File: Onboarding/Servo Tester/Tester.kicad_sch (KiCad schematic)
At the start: 6 parts, among them SW1 RotaryEncoder_Switch, U1 PCF8551ATT_AJ, U3 ATTINY204-SSNR, U4 AP2205-33Y-13, U5 VIM-878-DP-FC-S-LV

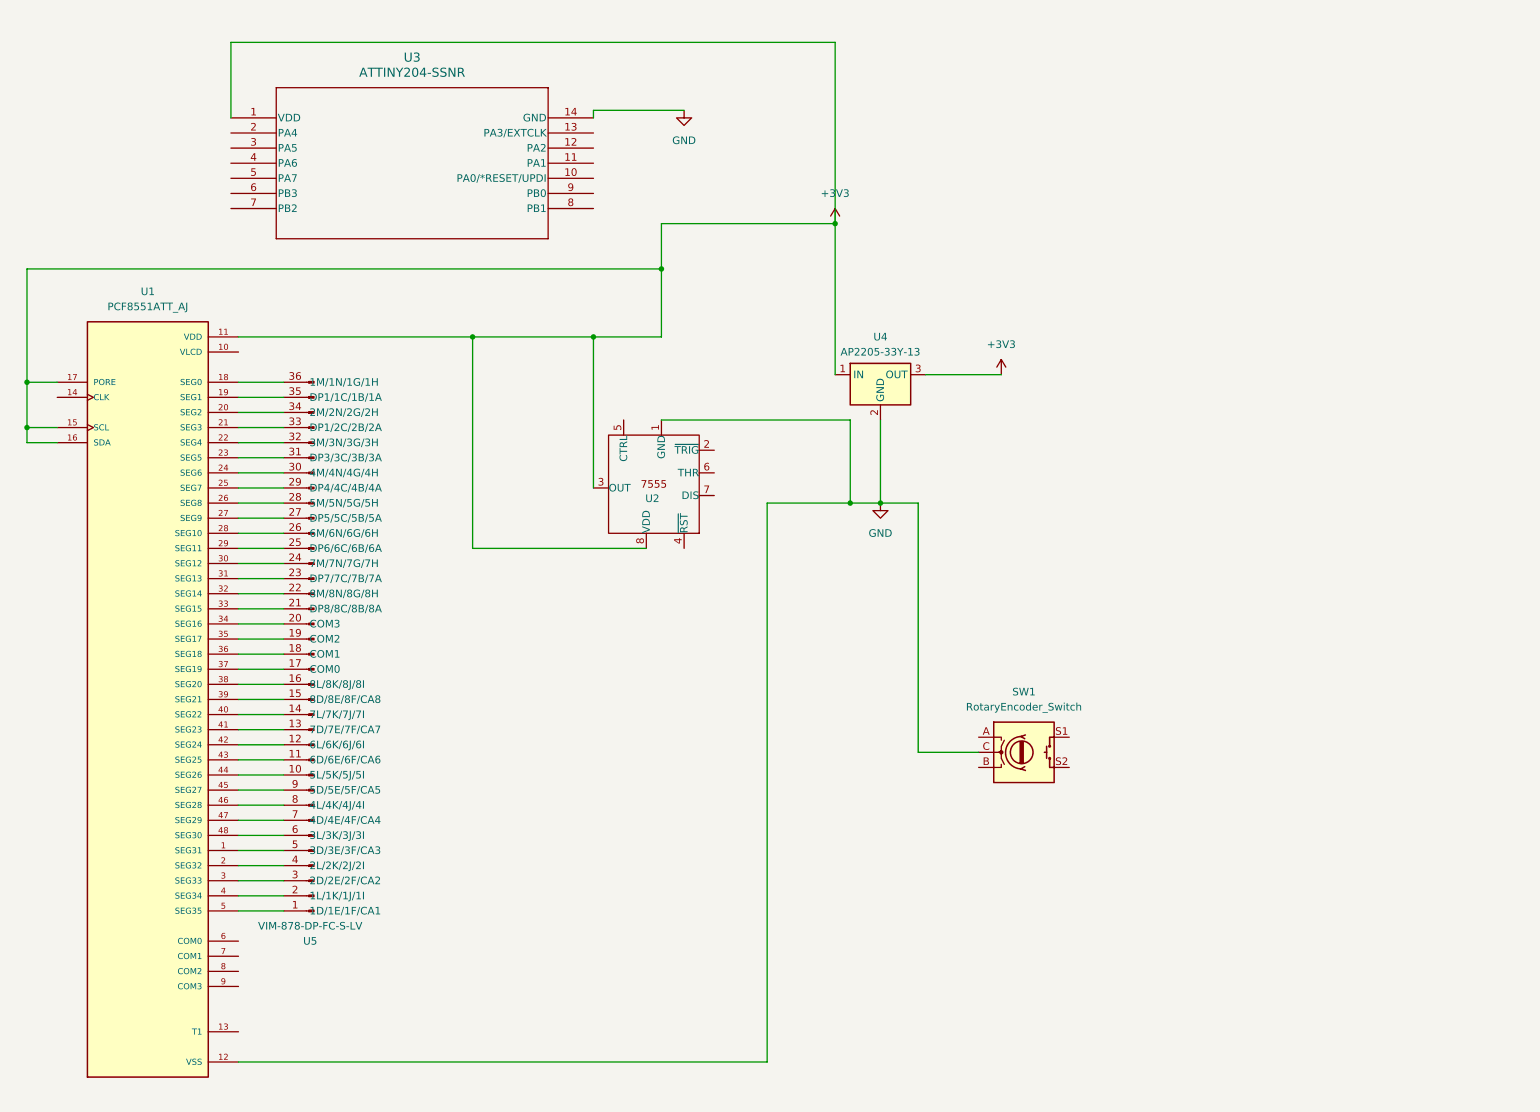
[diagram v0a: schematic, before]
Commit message: Update Tester.kicad_sch
Progress has been made.
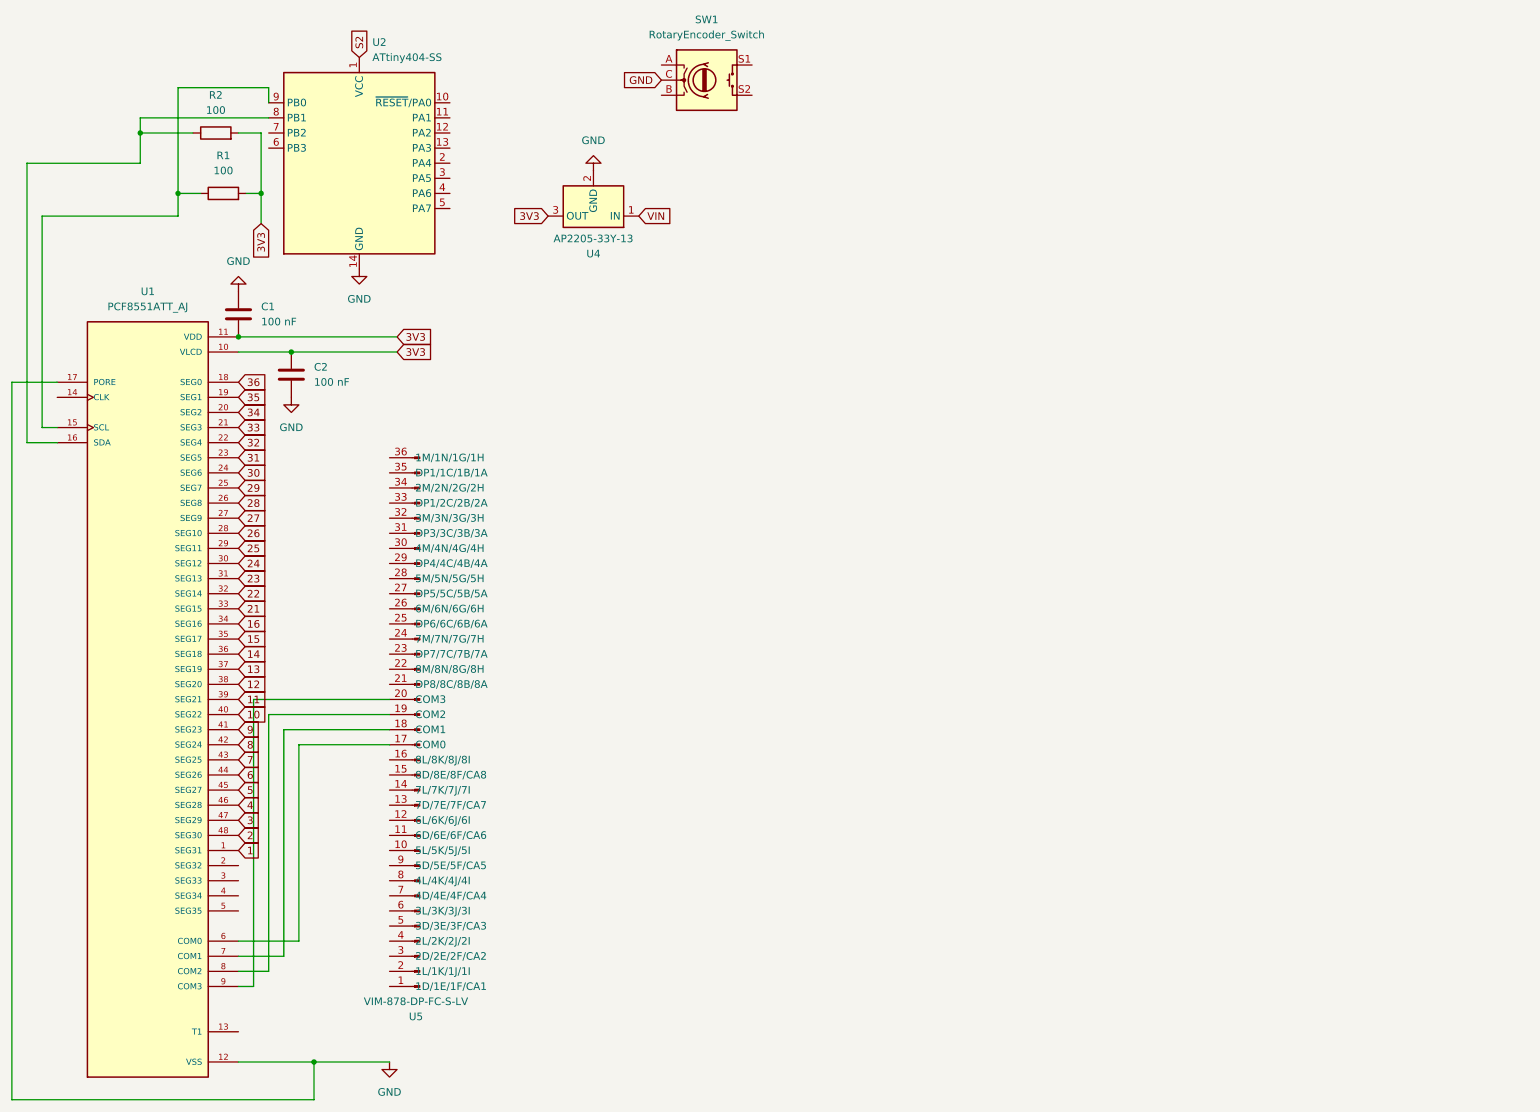
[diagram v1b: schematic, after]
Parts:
- removed U2: ~, symbol NewSymbolLibrary:7555
- removed U3: ATTINY204-SSNR, SOIC14_SL_MCH, symbol ServoTester:ATTINY204-SSNR
- added C1, C2: 100 nF, symbol Device:C
- added R1, R2: 100, symbol Device:R
- added U2: ATtiny404-SS, Package_SO:SOIC-14_3.9x8.7mm_P1.27mm, symbol servo_tester_onboarding:ATtiny404-SS
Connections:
- net GND: now also U1.17 (PORE), C1.1, C2.2, U2.14 (GND)
- net at U5.5 (3D/3E/3F/CA3): no longer U1.1 (SEG31)
- net 3V3: now reaches U1.10 (VLCD)
- net 3V3: now also U1.11 (VDD), U4.3 (OUT), C1.2, C2.1, R1.2, R2.2
- net at U5.36 (1M/1N/1G/1H): no longer U1.18 (SEG0)
- net at U5.35 (DP1/1C/1B/1A): no longer U1.19 (SEG1)
- net at U1.2 (SEG32): no longer U5.4 (2L/2K/2J/2I)
- net at U5.34 (2M/2N/2G/2H): no longer U1.20 (SEG2)
- net at U5.33 (DP1/2C/2B/2A): no longer U1.21 (SEG3)
- net at U5.32 (3M/3N/3G/3H): no longer U1.22 (SEG4)
- net at U5.31 (DP3/3C/3B/3A): no longer U1.23 (SEG5)
- net at U5.30 (4M/4N/4G/4H): no longer U1.24 (SEG6)
- net at U5.29 (DP4/4C/4B/4A): no longer U1.25 (SEG7)
- net at U5.28 (5M/5N/5G/5H): no longer U1.26 (SEG8)
- net at U5.27 (DP5/5C/5B/5A): no longer U1.27 (SEG9)
- net at U5.26 (6M/6N/6G/6H): no longer U1.28 (SEG10)
- net at U5.25 (DP6/6C/6B/6A): no longer U1.29 (SEG11)
- net at U1.3 (SEG33): no longer U5.3 (2D/2E/2F/CA2)
- net at U5.24 (7M/7N/7G/7H): no longer U1.30 (SEG12)
- net at U5.23 (DP7/7C/7B/7A): no longer U1.31 (SEG13)
- net at U5.22 (8M/8N/8G/8H): no longer U1.32 (SEG14)
- net at U5.21 (DP8/8C/8B/8A): no longer U1.33 (SEG15)
- net at U5.20 (COM3): now also U1.9 (COM3); no longer U1.34 (SEG16)
- net at U5.19 (COM2): now also U1.8 (COM2); no longer U1.35 (SEG17)
- net at U5.18 (COM1): now also U1.7 (COM1); no longer U1.36 (SEG18)
- net at U5.17 (COM0): now also U1.6 (COM0); no longer U1.37 (SEG19)
- net at U5.16 (8L/8K/8J/8I): no longer U1.38 (SEG20)
- net at U5.15 (8D/8E/8F/CA8): no longer U1.39 (SEG21)
- net at U1.4 (SEG34): no longer U5.2 (1L/1K/1J/1I)
- net at U5.14 (7L/7K/7J/7I): no longer U1.40 (SEG22)
- net at U5.13 (7D/7E/7F/CA7): no longer U1.41 (SEG23)
- net at U5.12 (6L/6K/6J/6I): no longer U1.42 (SEG24)
- net at U5.11 (6D/6E/6F/CA6): no longer U1.43 (SEG25)
- net at U5.10 (5L/5K/5J/5I): no longer U1.44 (SEG26)
- net at U5.9 (5D/5E/5F/CA5): no longer U1.45 (SEG27)
- net at U5.8 (4L/4K/4J/4I): no longer U1.46 (SEG28)
- net at U5.7 (4D/4E/4F/CA4): no longer U1.47 (SEG29)
- net at U5.6 (3L/3K/3J/3I): no longer U1.48 (SEG30)
- net at U1.5 (SEG35): no longer U5.1 (1D/1E/1F/CA1)
- removed net +3V3: U1.11 (VDD), U1.15 (SCL), U1.16 (SDA), U1.17 (PORE), U4.1 (IN), U4.3 (OUT)
- new net: R2.1, U1.16 (SDA), U2.8 (PB1)
- new net: R1.1, U1.15 (SCL), U2.9 (PB0)
- new net 1: U1.1 (SEG31)
- new net 10: U1.40 (SEG22)
- new net 11: U1.39 (SEG21)
- new net 12: U1.38 (SEG20)
- new net 13: U1.37 (SEG19)
- new net 14: U1.36 (SEG18)
- new net 15: U1.35 (SEG17)
- new net 16: U1.34 (SEG16)
- new net 2: U1.48 (SEG30)
- new net 21: U1.33 (SEG15)
- new net 22: U1.32 (SEG14)
- new net 23: U1.31 (SEG13)
- new net 24: U1.30 (SEG12)
- new net 25: U1.29 (SEG11)
- new net 26: U1.28 (SEG10)
- new net 27: U1.27 (SEG9)
- new net 28: U1.26 (SEG8)
- new net 29: U1.25 (SEG7)
- new net 3: U1.47 (SEG29)
- new net 30: U1.24 (SEG6)
- new net 31: U1.23 (SEG5)
- new net 32: U1.22 (SEG4)
- new net 33: U1.21 (SEG3)
- new net 34: U1.20 (SEG2)
- new net 35: U1.19 (SEG1)
- new net 36: U1.18 (SEG0)
- new net 4: U1.46 (SEG28)
- new net 5: U1.45 (SEG27)
- new net 6: U1.44 (SEG26)
- new net 7: U1.43 (SEG25)
- new net 8: U1.42 (SEG24)
- new net 9: U1.41 (SEG23)
- new net S2: U2.1 (VCC)
- new net VIN: U4.1 (IN)
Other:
- moved on the sheet: SW1, U4, U5

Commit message: Test_bat
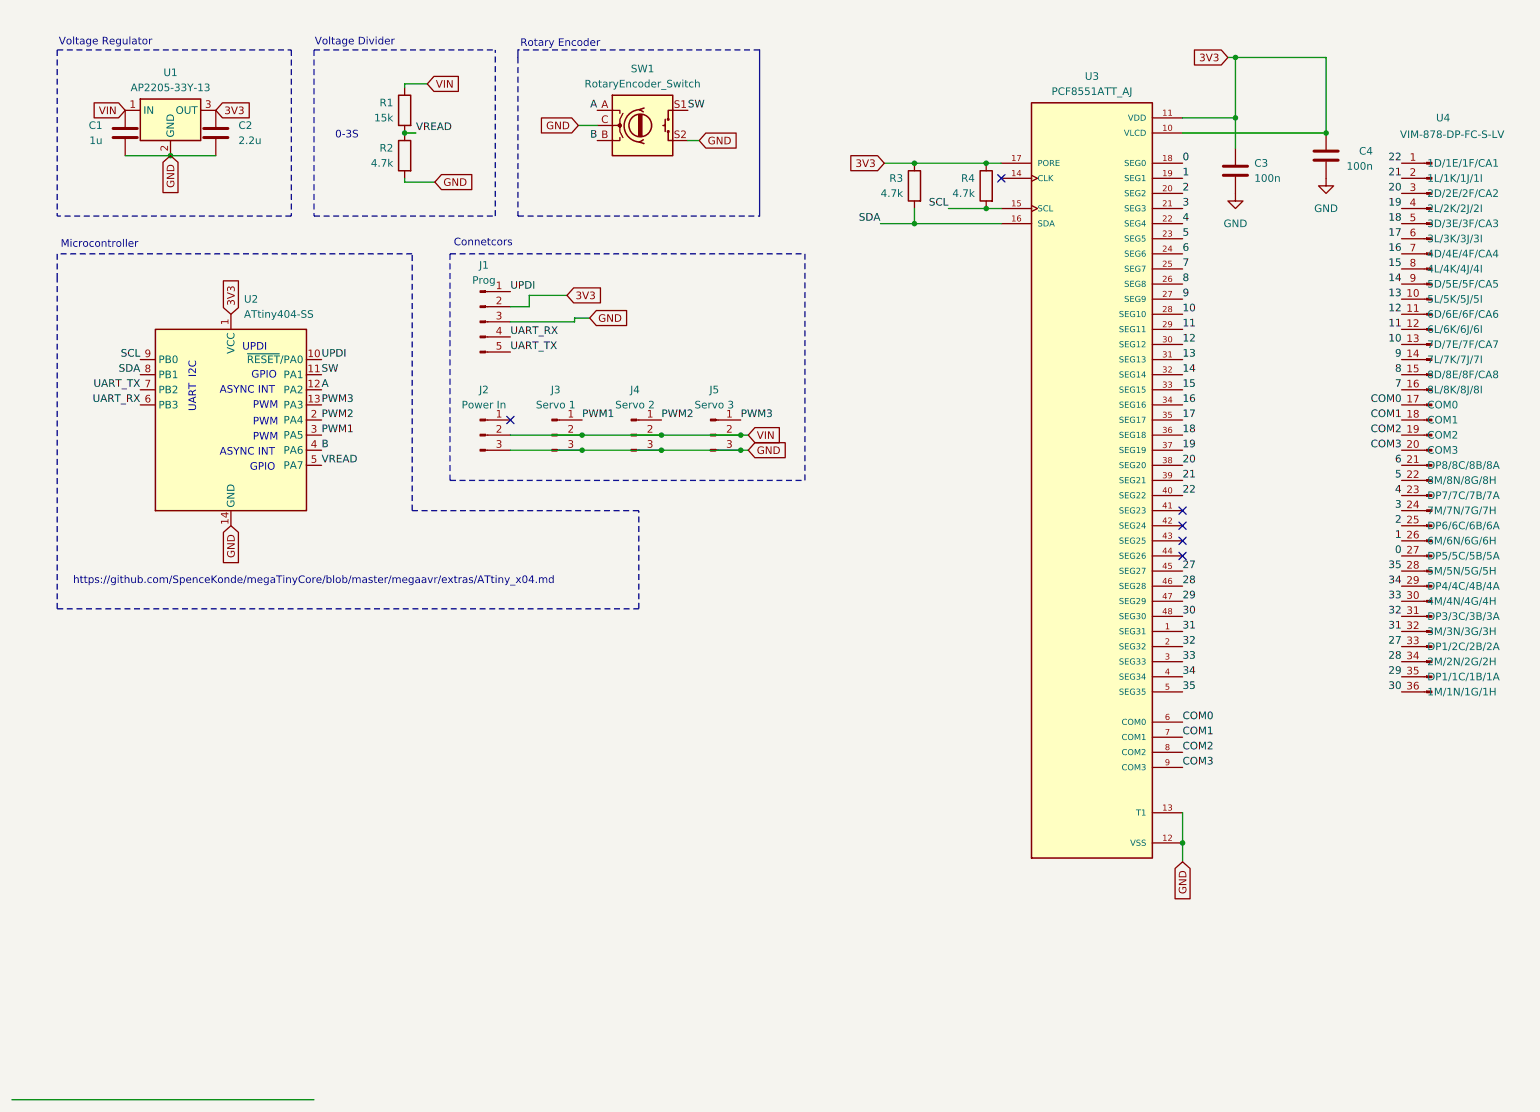
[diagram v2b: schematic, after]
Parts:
- removed SW1: RotaryEncoder_Switch, Rotary_Encoder:RotaryEncoder_Bourns_Vertical_PEC12R-3xxxF-Sxxxx, symbol servo_tester_onboarding:RotaryEncoder_Switch
- removed U1: PCF8551ATT_AJ, servo_tester:SOP50P810X120-48N, symbol servo_tester_onboarding:PCF8551ATT_AJ
- removed U2: ATtiny404-SS, Package_SO:SOIC-14_3.9x8.7mm_P1.27mm, symbol servo_tester_onboarding:ATtiny404-SS
- removed U4: AP2205-33Y-13, Package_TO_SOT_SMD:SOT-89-3_Handsoldering, symbol servo_tester_onboarding:AP2205-33Y-13
- removed U5: VIM-878-DP-FC-S-LV, symbol servo_tester_onboarding:VIM-878-DP
- added C3, C4: 100n, Capacitor_SMD:C_0603_1608Metric_Pad1.08x0.95mm_HandSolder, symbol Device:C
- added J1: Prog, Connector_PinSocket_2.54mm:PinSocket_1x05_P2.54mm_Vertical, symbol Connector:Conn_01x05_Pin
- added J2: Power In, Connector_PinSocket_2.54mm:PinSocket_1x03_P2.54mm_Vertical, symbol Connector:Conn_01x03_Pin
- added J3: Servo 1, Connector_PinSocket_2.54mm:PinSocket_1x03_P2.54mm_Vertical, symbol Connector:Conn_01x03_Pin
- added J4: Servo 2, Connector_PinSocket_2.54mm:PinSocket_1x03_P2.54mm_Vertical, symbol Connector:Conn_01x03_Pin
- added J5: Servo 3, Connector_PinSocket_2.54mm:PinSocket_1x03_P2.54mm_Vertical, symbol Connector:Conn_01x03_Pin
- added R3, R4: 4.7k, Resistor_SMD:R_0603_1608Metric_Pad0.98x0.95mm_HandSolder, symbol Device:R
- added SW1: RotaryEncoder_Switch, Rotary_Encoder:RotaryEncoder_Bourns_Vertical_PEC12R-3x17F-Sxxxx, symbol Device:RotaryEncoder_Switch
- added U1: AP2205-33Y-13, Package_TO_SOT_SMD:SOT-89-3_Handsoldering, symbol servo_tester:AP2205-33Y-13
- added U2: ATtiny404-SS, Package_SO:SOIC-14_3.9x8.7mm_P1.27mm, symbol MCU_Microchip_ATtiny:ATtiny404-SS
- added U3: PCF8551ATT_AJ, servo_tester:SOP50P810X120-48N, symbol servo_tester:PCF8551ATT_AJ
- added U4: VIM-878-DP-FC-S-LV, servo_tester:VIM-878-DP, symbol servo_tester:VIM-878-DP
- C1: value 100 nF -> 1u; footprint (none) -> Capacitor_SMD:C_0603_1608Metric_Pad1.08x0.95mm_HandSolder
- C2: value 100 nF -> 2.2u; footprint (none) -> Capacitor_SMD:C_0603_1608Metric_Pad1.08x0.95mm_HandSolder
- R1: value 100 -> 15k; footprint (none) -> Resistor_SMD:R_0603_1608Metric_Pad0.98x0.95mm_HandSolder
- R2: value 100 -> 4.7k; footprint (none) -> Resistor_SMD:R_0603_1608Metric_Pad0.98x0.95mm_HandSolder
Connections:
- net 1: now also U3.19 (SEG1), U4.26 (6M/6N/6G/6H)
- net 10: now also U3.28 (SEG10), U4.13 (7D/7E/7F/CA7)
- net 11: now also U3.29 (SEG11), U4.12 (6L/6K/6J/6I)
- net 12: now also U3.30 (SEG12), U4.11 (6D/6E/6F/CA6)
- net 13: now also U3.31 (SEG13), U4.10 (5L/5K/5J/5I)
- net 14: now also U3.32 (SEG14), U4.9 (5D/5E/5F/CA5)
- net 15: now also U3.33 (SEG15), U4.8 (4L/4K/4J/4I)
- net 16: now also U3.34 (SEG16), U4.7 (4D/4E/4F/CA4)
- net 2: now also U3.20 (SEG2), U4.25 (DP6/6C/6B/6A)
- net 21: now also U3.39 (SEG21), U4.2 (1L/1K/1J/1I)
- net 22: now also U3.40 (SEG22), U4.1 (1D/1E/1F/CA1)
- net 27: now also U3.45 (SEG27), U4.33 (DP1/2C/2B/2A)
- net 28: now also U3.46 (SEG28), U4.34 (2M/2N/2G/2H)
- net 29: now also U3.47 (SEG29), U4.35 (DP1/1C/1B/1A)
- net 3: now also U3.21 (SEG3), U4.24 (7M/7N/7G/7H)
- net 30: now also U3.48 (SEG30), U4.36 (1M/1N/1G/1H)
- net 31: now also U3.1 (SEG31), U4.32 (3M/3N/3G/3H)
- net 32: now also U3.2 (SEG32), U4.31 (DP3/3C/3B/3A)
- net 33: now also U3.3 (SEG33), U4.30 (4M/4N/4G/4H)
- net 34: now also U3.4 (SEG34), U4.29 (DP4/4C/4B/4A)
- net 35: now also U3.5 (SEG35), U4.28 (5M/5N/5G/5H)
- net 3V3: now also C3.1, C4.1, J1.2 (Pin_2), R3.1, R4.1, U1.3 (OUT), U2.1 (VCC), U3.10 (VLCD), U3.11 (VDD), U3.17 (PORE); no longer C1.2, R1.2, R2.2
- net 4: now also U3.22 (SEG4), U4.23 (DP7/7C/7B/7A)
- net 5: now also U3.23 (SEG5), U4.22 (8M/8N/8G/8H)
- net 6: now also U3.24 (SEG6), U4.21 (DP8/8C/8B/8A)
- net 7: now also U3.25 (SEG7), U4.16 (8L/8K/8J/8I)
- net 8: now also U3.26 (SEG8), U4.15 (8D/8E/8F/CA8)
- net 9: now also U3.27 (SEG9), U4.14 (7L/7K/7J/7I)
- net GND: now also C1.2, R2.2, C3.2, C4.2, J1.3 (Pin_3), J2.3 (Pin_3), J3.3 (Pin_3), J4.3 (Pin_3), J5.3 (Pin_3), SW1.C, SW1.S2, U1.2 (GND), U2.14 (GND), U3.12 (VSS), U3.13 (T1); no longer C1.1
- net VIN: now also C1.1, R1.1, J2.2 (Pin_2), J3.2 (Pin_2), J4.2 (Pin_2), J5.2 (Pin_2), U1.1 (IN)
- net VREAD: now reaches R2.1
- net VREAD: now also R1.2, U2.5 (PA7)
- new net 0: U3.18 (SEG0), U4.27 (DP5/5C/5B/5A)
- new net 17: U3.35 (SEG17), U4.6 (3L/3K/3J/3I)
- new net 18: U3.36 (SEG18), U4.5 (3D/3E/3F/CA3)
- new net 19: U3.37 (SEG19), U4.4 (2L/2K/2J/2I)
- new net 20: U3.38 (SEG20), U4.3 (2D/2E/2F/CA2)
- new net A: SW1.A, U2.12 (PA2)
- new net B: SW1.B, U2.4 (PA6)
- new net COM0: U3.6 (COM0), U4.17 (COM0)
- new net COM1: U3.7 (COM1), U4.18 (COM1)
- new net COM2: U3.8 (COM2), U4.19 (COM2)
- new net COM3: U3.9 (COM3), U4.20 (COM3)
- new net PWM1: J3.1 (Pin_1), U2.3 (PA5)
- new net PWM2: J4.1 (Pin_1), U2.2 (PA4)
- new net PWM3: J5.1 (Pin_1), U2.13 (PA3)
- new net SCL: R4.2, U2.9 (PB0), U3.15 (SCL)
- new net SDA: R3.2, U2.8 (PB1), U3.16 (SDA)
- new net SW: SW1.S1, U2.11 (PA1)
- new net UART_RX: J1.4 (Pin_4), U2.6 (PB3)
- new net UART_TX: J1.5 (Pin_5), U2.7 (PB2)
- new net UPDI: J1.1 (Pin_1), U2.10 (~{RESET}/PA0)
- no-connect marks 0 -> 6
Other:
- note added: "0-3S"
- note added: "ASYNC INT"
- note added: "Connetcors"
- note added: "GPIO"
- note added: "I2C"
- note added: "Microcontroller"
- note added: "PWM"
- note added: "Rotary Encoder"
- note added: "UART"
- note added: "UPDI"
- note added: "Voltage Divider"
- note added: "Voltage Regulator"
- note added: "https://github.com/SpenceKonde/megaTinyCore/blob/master/megaavr/extras/ATtiny_x04.md"
